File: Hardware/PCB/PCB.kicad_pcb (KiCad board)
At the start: 2 copper layers, 63 parts, among them J1 USB_C_Receptacle_PowerOnly_6P, J2 I2C_SSD1306, J3 USB_C_Receptacle_PowerOnly_6P, J4 53048-0510, Q1 DMN33D8LT-7, Q2 NMOS, Q3 PJC138K_R1_00001, Q4 PJC138K_R1_00001, SW1 SW_HotSwap, U1 MCP98243, U2 LP2985-3.3, U3 STM32F303RETx, U4 MC1413BD, U5 USBLC6-2P6, U6 USBLC6-2P6, U7 FT231XQ, U8 MPU-9250, X1 ECS-2520MV-250-DN-TR

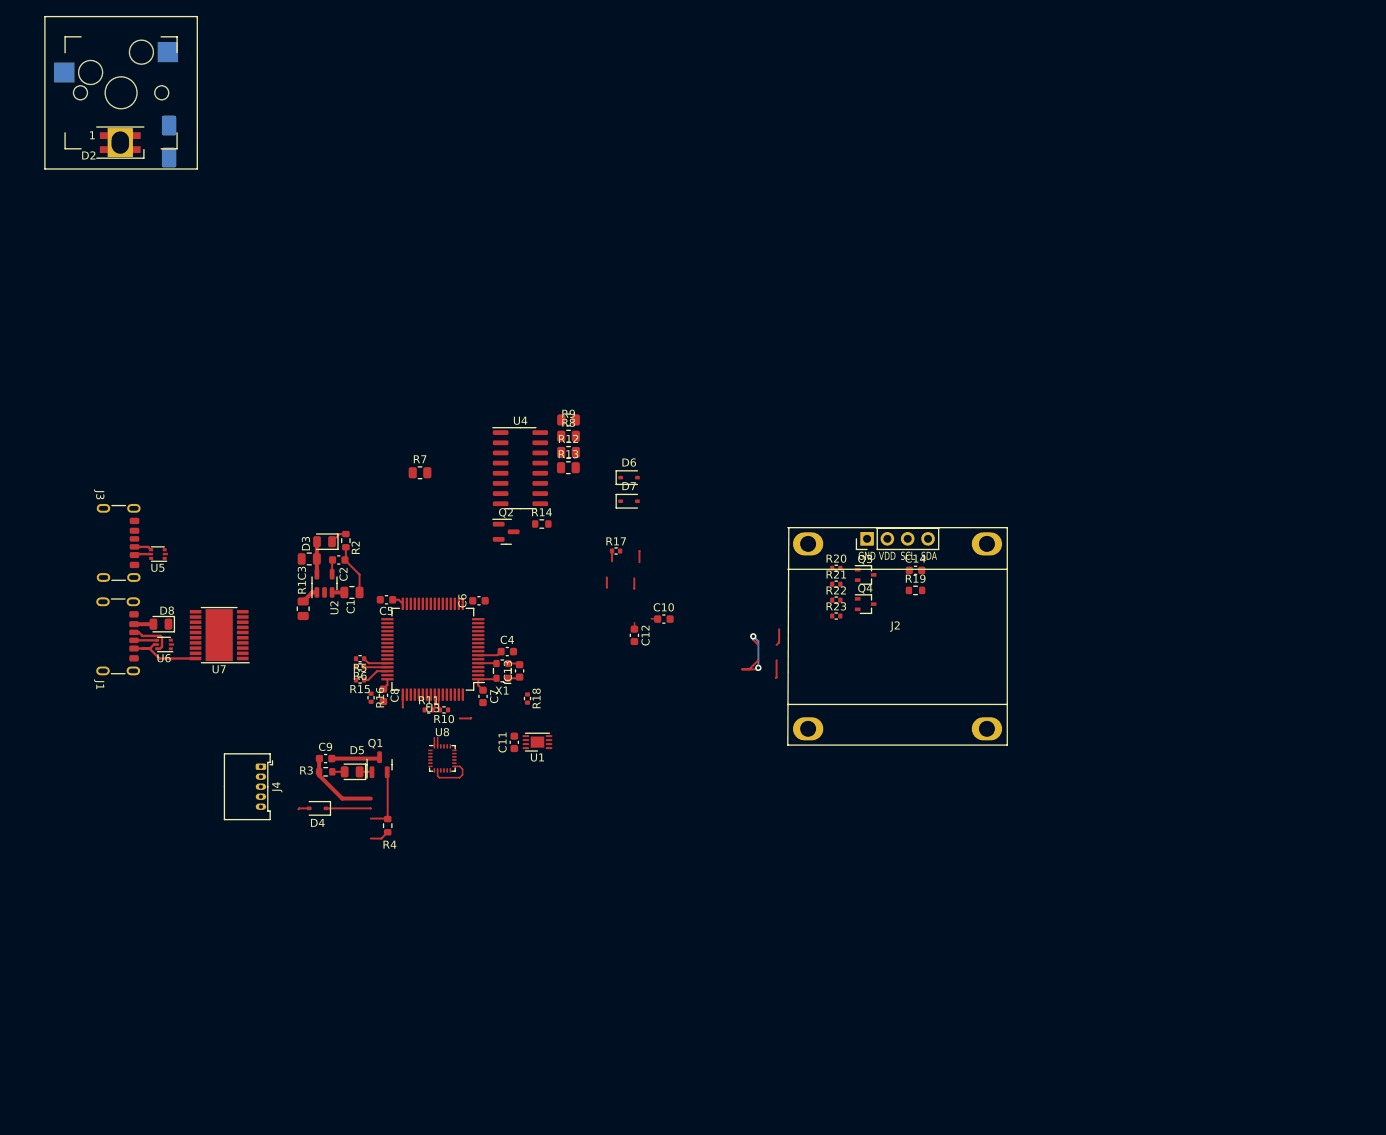
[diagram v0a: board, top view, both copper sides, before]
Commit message: update of directory
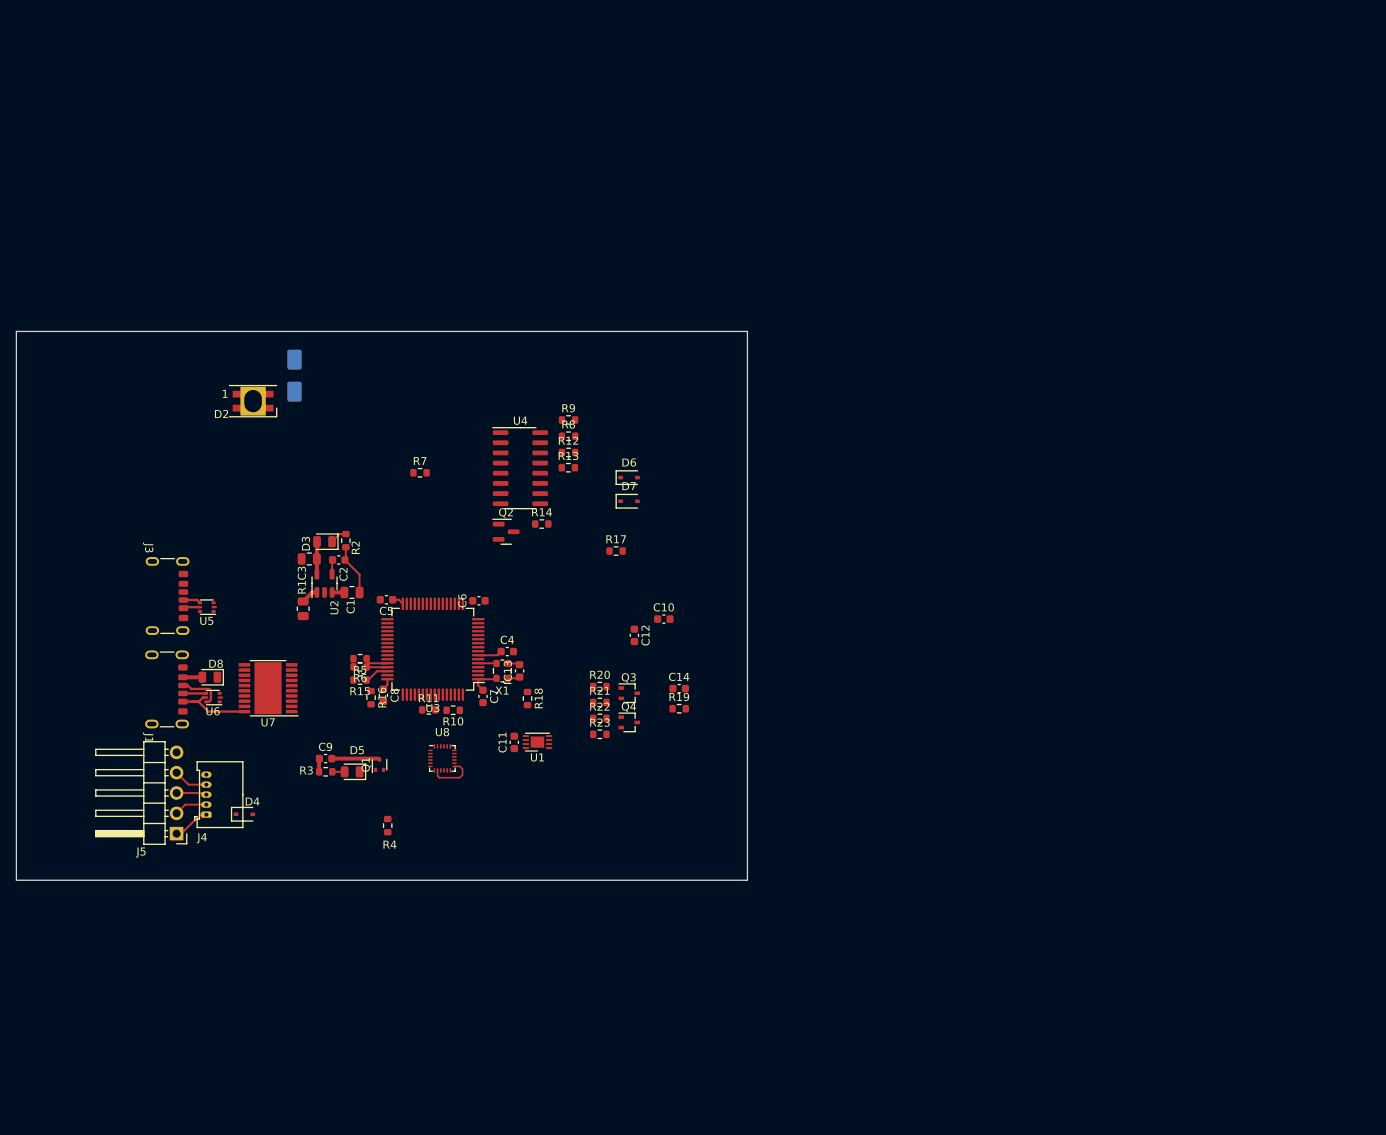
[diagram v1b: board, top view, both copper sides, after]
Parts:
- removed J2: I2C_SSD1306, OLED:SSD1306_OLED_Display(128x64)
- removed SW1: SW_HotSwap, HotSwapp_1U:Hotswap_1U
- added J5: Pin_Header, Connector_PinHeader_2.54mm:PinHeader_1x05_P2.54mm_Horizontal, F.Cu at (133.3, 136.7)
- C1: value 2.2uF -> 4.7uF
- C2: value 10nF -> 100nF
- D2: value SK6812MINI -> SK6812MINI-E
- Q1: footprint Package_TO_SOT_SMD:SOT-23 -> Package_TO_SOT_SMD:SOT-523
- R10, R11, R15, R16, R17, R18, R20, R21, R22, R23, R5, R6: footprint Resistor_SMD:R_0402_1005Metric -> Resistor_SMD:R_0603_1608Metric
- R12, R13, R7, R8, R9: footprint Resistor_SMD:R_0805_2012Metric -> Resistor_SMD:R_0603_1608Metric
- moved D2 36.3 mm to (142.8, 82.6)
- moved D1 33.2 mm to (148.0, 79.4), turned to 90 degrees
- moved C14 33.0 mm to (196.1, 118.5)
- moved R19 33.0 mm to (196.1, 121.1)
- moved R20 33.0 mm to (186.2, 118.3)
- moved R21 33.0 mm to (186.2, 120.3)
- moved R22 33.0 mm to (186.2, 122.3)
- moved R23 33.0 mm to (186.2, 124.3)
- moved Q3 33.0 mm to (189.9, 119.1)
- moved Q4 33.0 mm to (189.9, 122.8)
- moved D4 9.18 mm to (141.8, 134.2), turned to 0 degrees
- moved J4 9.07 mm to (137.0, 134.3), turned to 90 degrees
- moved J1 9.02 mm to (131.0, 118.7)
- moved U7 9.02 mm to (144.7, 118.5)
- moved J3 9.02 mm to (131.1, 107.0)
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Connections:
- Q3 pad 2: /OLED/+3.3V -> /IMU/+3.3V
- Q4 pad 2: /OLED/+3.3V -> /IMU/+3.3V
- R22 pad 2: /OLED/+3.3V -> /IMU/+3.3V
- R23 pad 2: /OLED/+3.3V -> /IMU/+3.3V
- U3 pad 42: unconnected-(U3-PA9-Pad42) -> /MCU/TX
- U3 pad 43: unconnected-(U3-PA10-Pad43) -> /MCU/RX
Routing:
- net Net-(U2-ON/~{OFF}): track 13.9 -> 3.71 mm, vias 2 -> 0
- net (no net): track 6.95 -> 0.00 mm
- net /IMU/SCL: track 4.85 -> 0.00 mm
- net /MCU/SWD: track 8.02 -> 3.81 mm
- net /MCU/SWC: track 0.00 -> 4.17 mm
- net /USB_Slot/VBus: track 11.8 -> 8.06 mm
- net /IMU/+3.3V: track 22.0 -> 18.4 mm
- net /IMU/SDA: track 3.10 -> 0.00 mm
- net GND: track 16.4 -> 13.7 mm
- net Net-(U3-PA14): track 1.61 -> 0.00 mm
- net Net-(D5-K): track 1.56 -> 0.00 mm
- net /MCU/NRST: track 4.46 -> 3.05 mm
- net /UART_Slot/VBus: track 13.9 -> 12.6 mm
- net Net-(D4-K): track 5.61 -> 4.71 mm
- net Net-(U3-PA13): track 3.36 -> 2.86 mm
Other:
- board outline added: 91.4 x 68.6 mm
- board text added: "PCB3D_BR_PCBA"
- board text added: "PCB3D_TL_PCBA"

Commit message: save
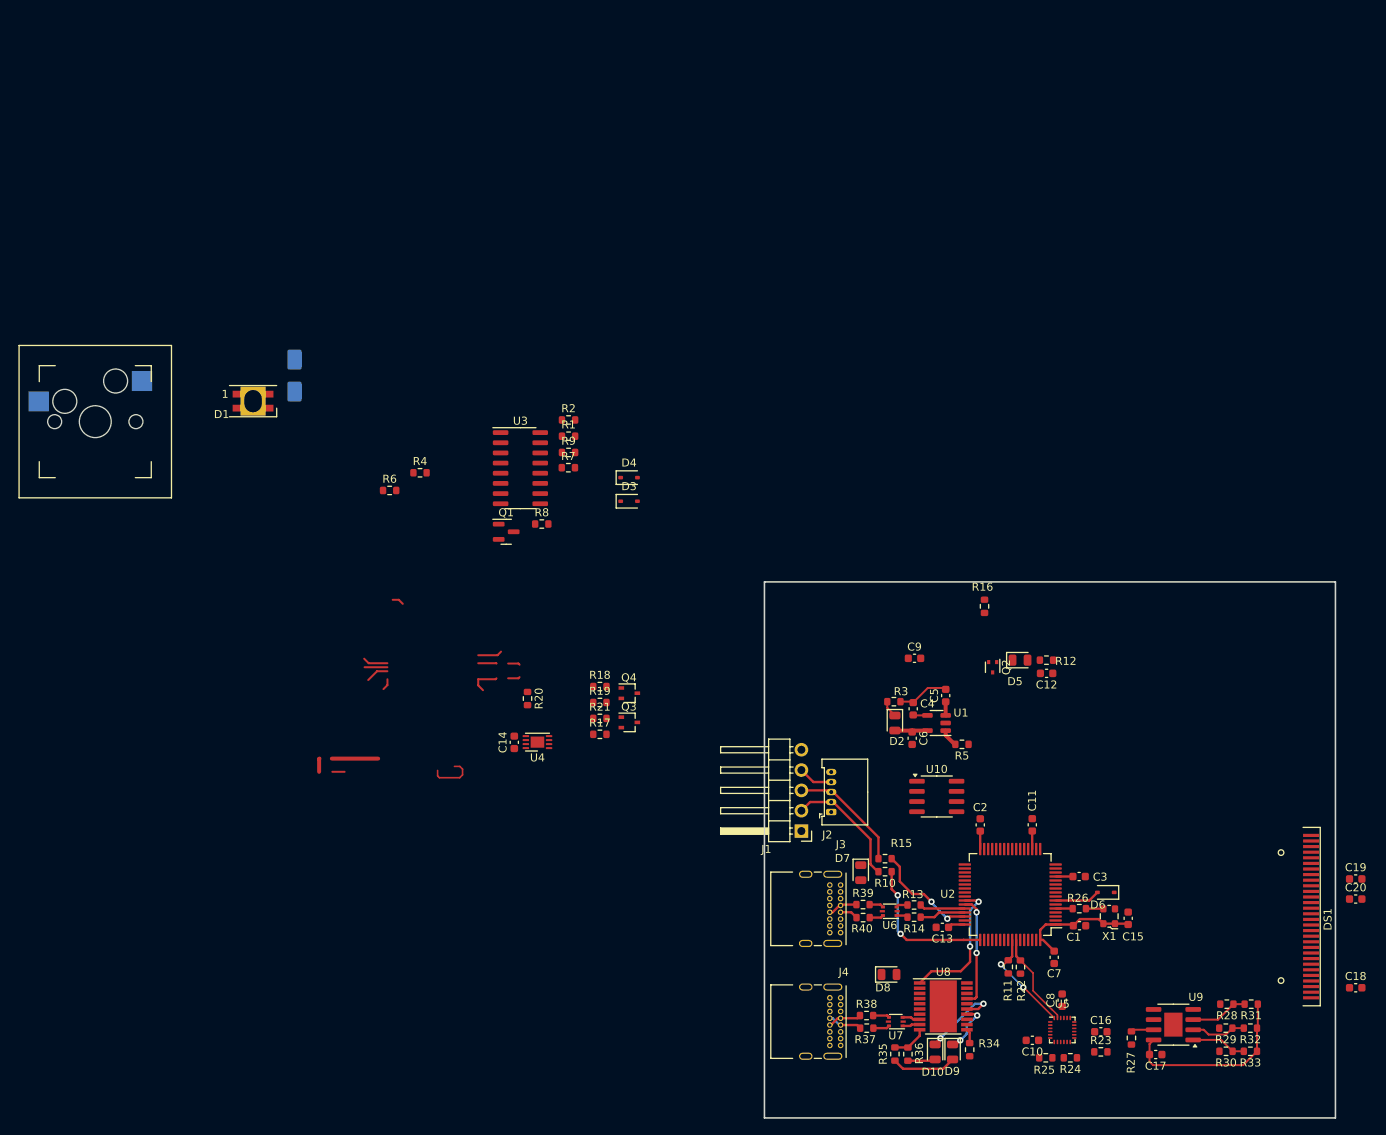
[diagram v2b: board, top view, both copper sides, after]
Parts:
- removed the J3 at (131.1, 107.0)
- added C1: 100nF, Capacitor_SMD:C_0603_1608Metric, F.Cu at (246.1, 148.2)
- added C17: 100nF, Capacitor_SMD:C_0603_1608Metric, F.Cu at (255.7, 164.3)
- added C18: 4.7uF, Capacitor_SMD:C_0603_1608Metric, F.Cu at (280.7, 155.9)
- added C19: 1µF, Capacitor_SMD:C_0603_1608Metric, F.Cu at (280.7, 142.3)
- added C2: 100nF, Capacitor_SMD:C_0603_1608Metric, F.Cu at (233.7, 135.6)
- added C20: 1µF, Capacitor_SMD:C_0603_1608Metric, F.Cu at (280.7, 144.9)
- added D10: LED, LED_SMD:LED_0805_2012Metric, F.Cu at (228.1, 164.0)
- added D7: D, Diode_SMD:D_0805_2012Metric, F.Cu at (218.8, 141.6)
- added D9: LED, LED_SMD:LED_0805_2012Metric, F.Cu at (230.3, 164.0)
- added DS1: OLED-128O064D, Display:OLED-128O064D, F.Cu at (275.1, 147.0)
- added J4: USB_C_Receptacle_USB2.0_16P, Connector_USB:USB_C_Receptacle_GCT_USB4085, F.Cu at (216.3, 157.2)
- added R24: 10k, Resistor_SMD:R_0603_1608Metric, F.Cu at (245.0, 164.7)
- added R25: 10k, Resistor_SMD:R_0603_1608Metric, F.Cu at (241.9, 164.7)
- added R26: 10, Resistor_SMD:R_0603_1608Metric, F.Cu at (246.1, 146.1)
- added R27: 10k, Resistor_SMD:R_0603_1608Metric, F.Cu at (252.6, 162.2)
- added R28: 10k, Resistor_SMD:R_0603_1608Metric, F.Cu at (264.6, 158.0)
- added R29: 10k, Resistor_SMD:R_0603_1608Metric, F.Cu at (264.4, 161.0)
- added R30: 10k, Resistor_SMD:R_0603_1608Metric, F.Cu at (264.5, 163.9)
- added R31: 10k, Resistor_SMD:R_0603_1608Metric, F.Cu at (267.6, 158.0)
- added R32: 10k, Resistor_SMD:R_0603_1608Metric, F.Cu at (267.5, 161.0)
- added R33: 10k, Resistor_SMD:R_0603_1608Metric, F.Cu at (267.5, 163.9)
- added R35: 270, Resistor_SMD:R_0603_1608Metric, F.Cu at (223.1, 164.2)
- added R36: 270, Resistor_SMD:R_0603_1608Metric, F.Cu at (224.7, 164.2)
- added R37: 22, Resistor_SMD:R_0603_1608Metric, F.Cu at (219.5, 161.0)
- added R38: 22, Resistor_SMD:R_0603_1608Metric, F.Cu at (219.5, 159.4)
- added R39: 22, Resistor_SMD:R_0603_1608Metric, F.Cu at (219.1, 145.5)
- added R40: 22, Resistor_SMD:R_0603_1608Metric, F.Cu at (219.1, 147.2)
- added R6: 0, Resistor_SMD:R_0603_1608Metric, F.Cu at (159.9, 93.8)
- added SW1: SW_HotSwap, HotSwapp_1U:Hotswap_1U, F.Cu at (123.1, 85.2)
- added U10: ACS712xLCTR-05B, Package_SO:SOIC-8_3.9x4.9mm_P1.27mm, F.Cu at (228.3, 132.0)
- added U9: 24LC64, Package_SO:SOIC-8-1EP_3.9x4.9mm_P1.27mm_EP2.29x3mm, F.Cu at (257.9, 160.6)
- C5: renamed from C1; footprint Capacitor_SMD:C_0805_2012Metric -> Capacitor_SMD:C_0603_1608Metric
- C6: renamed from C3; footprint Capacitor_SMD:C_0805_2012Metric -> Capacitor_SMD:C_0603_1608Metric
- C7: renamed from C6; value 470nF -> 100nF
- J3: renamed from J1; value USB_C_Receptacle_PowerOnly_6P -> USB_C_Receptacle_USB2.0_16P; footprint Connector_USB:USB_C_Receptacle_GCT_USB4125-xx-x_6P_TopMnt_Horizontal -> Connector_USB:USB_C_Receptacle_GCT_USB4085
- R23: renamed from R19; value 47k -> 10k
- R5: renamed from R1; value 18 -> 270; footprint Resistor_SMD:R_0805_2012Metric -> Resistor_SMD:R_0603_1608Metric
- moved D6 108.1 mm to (249.4, 144.0), turned to 180 degrees
- moved U7 94.5 mm to (223.2, 160.2)
- moved U6 93.4 mm to (222.4, 146.4)
- moved U8 93.3 mm to (229.1, 158.3), turned to 0 degrees
- moved C3 93.2 mm to (246.1, 142.0), turned to 0 degrees
- moved D8 92.7 mm to (222.3, 154.3), turned to 0 degrees
- moved R12 91.2 mm to (242.0, 115.0), turned to 180 degrees
- moved C12 90.7 mm to (242.0, 116.6), turned to 180 degrees
- moved J3 88.7 mm to (216.3, 143.1)
- moved D5 84.6 mm to (238.7, 115.0), turned to 0 degrees
- moved C7 84.6 mm to (243.0, 152.1), turned to -90 degrees
- moved U5 84.6 mm to (244.0, 161.2)
- moved R5 84.1 mm to (231.4, 125.5), turned to 180 degrees
- moved C11 82.7 mm to (240.2, 135.6), turned to 90 degrees
- moved C15 82.1 mm to (252.2, 147.3)
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- renumbered C8 to C11, C9 to C12, C7 to C13, C11 to C14, C13 to C15, C14 to C16, C5 to C3, C2 to C4, C12 to C8, C4 to C9, D2 to D1, D1 to D11, D3 to D2, D7 to D3, D6 to D4, D4 to D6, J5 to J1, J4 to J2, Q2 to Q1, Q1 to Q2, Q4 to Q3, Q3 to Q4, R8 to R1, R16 to R10, R3 to R12, R5 to R13, R6 to R14, R4 to R16, R23 to R17, R20 to R18, R21 to R19, R9 to R2, R18 to R20, R22 to R21, R10 to R22, R2 to R3, R17 to R34, R7 to R4, R13 to R7, R14 to R8, R12 to R9, U2 to U1, U3 to U2, U4 to U3, U1 to U4, U8 to U5, U5 to U6, U6 to U7, U7 to U8
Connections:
- C12 pad 1: /USB_Slot/VBus -> /Programming/+5V_OUT
- C4 pad 2: GND -> /Supply/GND
- C5 pad 1: Net-(U2-ON/~{OFF}) -> Net-(U1-ON/~{OFF})
- C5 pad 2: GND -> /Supply/GND
- C6 pad 2: GND -> /Supply/GND
- D8 pad 1: /USB_Slot/VBus -> /Programming/+5V_OUT
- J1 pad 4: /USB_Slot/VBus -> /Programming/+5V_OUT
- J2 pad 4: /USB_Slot/VBus -> /Programming/+5V_OUT
- J3 pad A5: Net-(J1-CC1) -> unconnected-(J3-CC1-PadA5)
- J3 pad A9: /UART_Slot/VBus -> /USB_Slot/VBus
- J3 pad B5: Net-(J1-CC2) -> unconnected-(J3-CC2-PadB5)
- J3 pad B9: /UART_Slot/VBus -> /USB_Slot/VBus
- R12 pad 1: /USB_Slot/VBus -> /Programming/+5V_OUT
- R3 pad 1: GND -> /Supply/GND
- R34 pad 1: /UART_Slot/VBus -> /UART_Slot/+3.3V
- R5 pad 1: /Multimeter/+5V -> Net-(U10-VIOUT)
- R5 pad 2: Net-(U2-ON/~{OFF}) -> /Supply/V_{CURRENT}
- U1 pad 1: Net-(U2-ON/~{OFF}) -> Net-(U1-ON/~{OFF})
- U1 pad 2: GND -> /Supply/GND
- U1 pad 3: Net-(U2-ON/~{OFF}) -> Net-(U1-ON/~{OFF})
- U2 pad 5: Net-(U3-PF0) -> Net-(U2-PF0)
- U2 pad 60: GND -> Net-(U2-BOOT0)
- U5 pad 1: /IMU/+3.3V -> unconnected-(U5-RESV_VDDIO-Pad1)
- U5 pad 9: unconnected-(U8-AD0/MISO-Pad9) -> Net-(U5-AD0/MISO)
- U6 pad 1: /MCU/USB+ -> /MCU/USB-
- U6 pad 3: /MCU/USB- -> /MCU/USB+
- U7 pad 1: Net-(U7-USBDP) -> Net-(U8-USBDM)
- U7 pad 2: unconnected-(U6-GND-Pad2) (its old number) -> GND
- U7 pad 3: Net-(U7-USBDM) -> Net-(U8-USBDP)
- U7 pad 4: Net-(J1-CC2) -> Net-(R38-Pad2)
- U7 pad 6: Net-(J1-CC1) -> Net-(R37-Pad2)
- U8 pad 10: unconnected-(U7-3V3OUT-Pad10) -> /UART_Slot/+3.3V
- U8 pad 13: unconnected-(U7-GND-Pad13) -> GND
- U8 pad 14: unconnected-(U7-CBUS1-Pad14) -> Net-(D9-K)
- U8 pad 15: unconnected-(U7-CBUS0-Pad15) -> Net-(D10-K)
- U8 pad 21: unconnected-(U7-GND-Pad21) -> GND
- U8 pad 3: unconnected-(U7-GND-Pad3) -> GND
- U8 pad 8: Net-(U7-USBDP) -> Net-(U8-USBDP)
- U8 pad 9: Net-(U7-USBDM) -> Net-(U8-USBDM)
- X1 pad 3: Net-(U3-PF0) -> Net-(X1-OUT)
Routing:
- net /IMU/+3.3V: track 18.4 -> 42.8 mm
- net /EEPROM/+3.3V: track 0.00 -> 23.2 mm
- net Net-(U2-PA14): track 0.00 -> 18.5 mm, vias 0 -> 2
- net /MCU/TX: track 0.00 -> 17.1 mm, vias 0 -> 2
- net /MCU/RX: track 0.00 -> 14.0 mm, vias 0 -> 2
- net /IMU/SDA: track 0.00 -> 13.4 mm, vias 0 -> 2
- net /UART_Slot/VBus: track 12.6 -> 0.00 mm
- net /IMU/SCL: track 0.00 -> 11.9 mm
- net /MCU/SWC: track 4.17 -> 15.5 mm
- net /MCU/SWD: track 3.81 -> 14.7 mm
- net Net-(U2-PA13): track 2.86 -> 13.5 mm, vias 0 -> 2
- net Net-(D10-K): track 0.00 -> 10.6 mm, vias 0 -> 2
- net (no net): track 0.00 -> 8.86 mm
- net Net-(D9-A): track 0.00 -> 8.12 mm
- net /USB_Slot/VBus: track 8.06 -> 0.00 mm
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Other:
- board size 91.4 x 68.6 mm -> 71.4 x 67 mm
- board text removed: "PCB3D_BR_PCBA"
- board text removed: "PCB3D_TL_PCBA"
